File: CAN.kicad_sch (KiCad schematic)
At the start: 8 parts, among them U1 TJA1051T-3

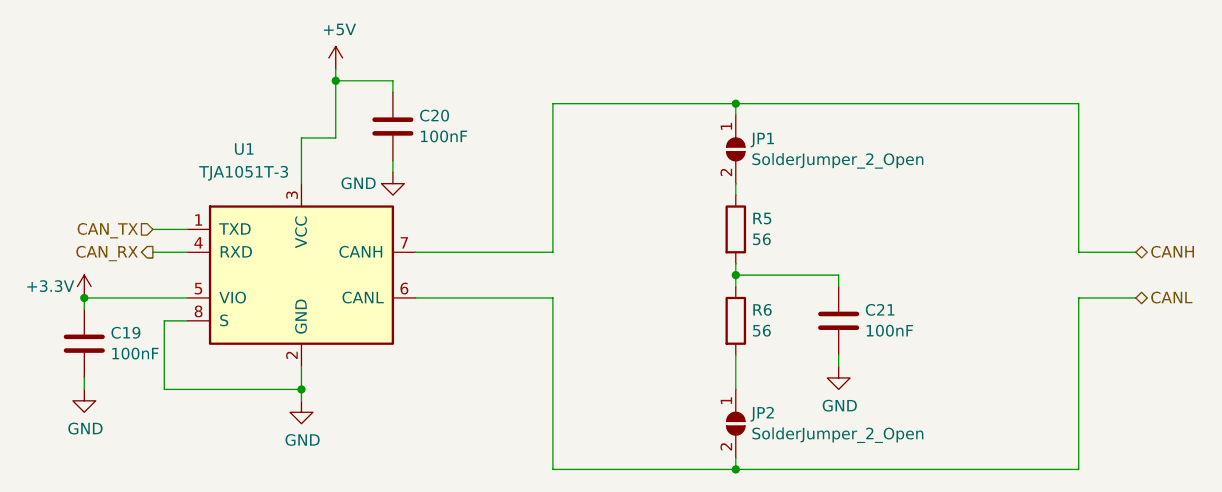
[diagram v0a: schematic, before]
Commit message: Add some decoupling caps; some more cleanups
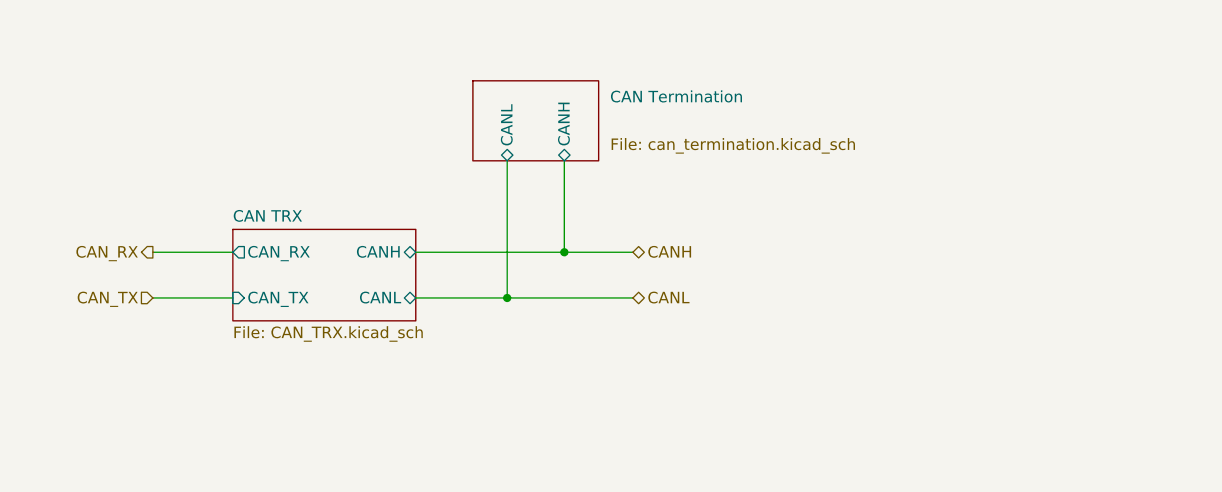
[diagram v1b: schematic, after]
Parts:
- removed C19, C20, C21: 100nF, Capacitor_SMD:C_0603_1608Metric, symbol Device:C
- removed JP1, JP2: SolderJumper_2_Open, Jumper:SolderJumper-2_P1.3mm_Open_RoundedPad1.0x1.5mm, symbol Jumper:SolderJumper_2_Open
- removed R5, R6: 56, Resistor_SMD:R_0603_1608Metric, symbol Device:R
- removed U1: TJA1051T-3, Package_SO:SOIC-8_3.9x4.9mm_P1.27mm, symbol Interface_CAN_LIN:TJA1051T-3
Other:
- added sheet CAN TRX (CAN_TRX.kicad_sch)
- added sheet CAN Termination (can_termination.kicad_sch)
